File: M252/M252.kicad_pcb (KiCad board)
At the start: 2 copper layers, 50 x 40 mm, 20 parts, among them IC101 PIC16F1827-I/P, J101 UART, J102 PROG, J103 TRIP, Q101 10MHz, SW101 !MCLR

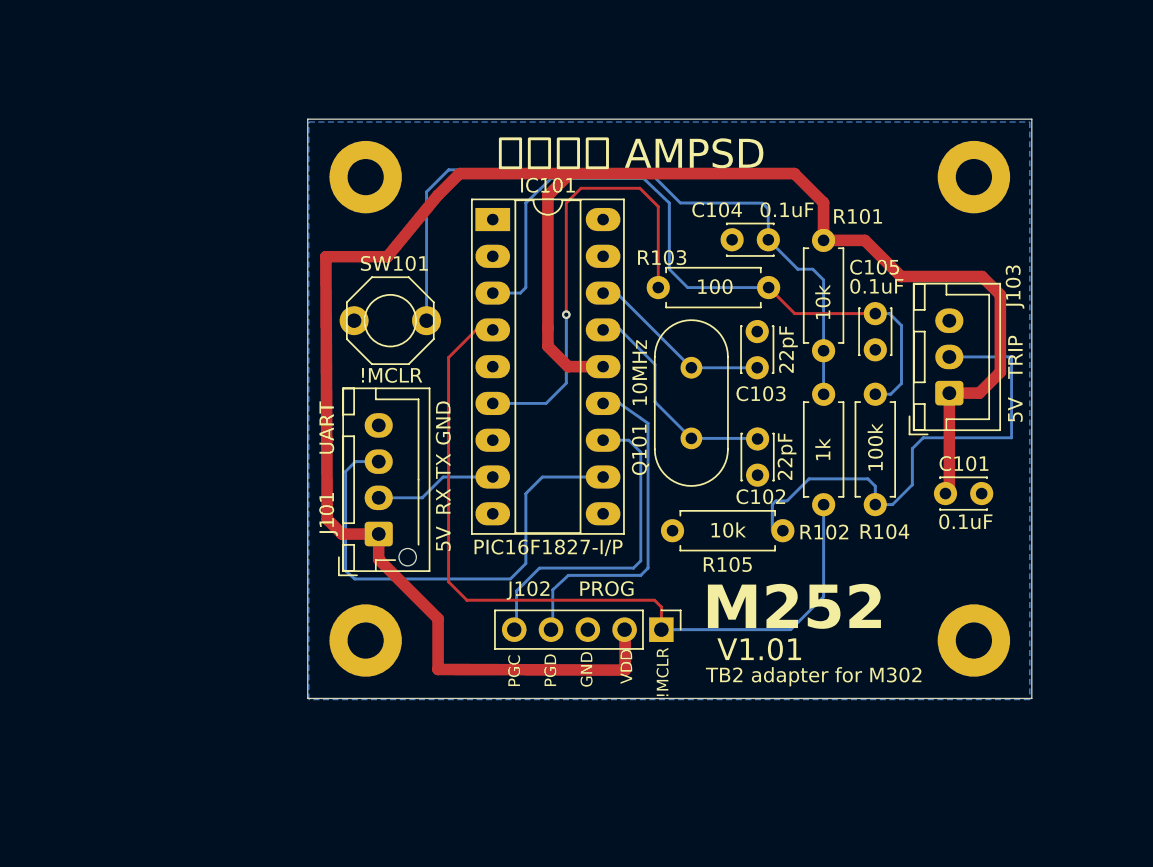
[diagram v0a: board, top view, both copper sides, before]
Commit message: UNO直結タイプ1st
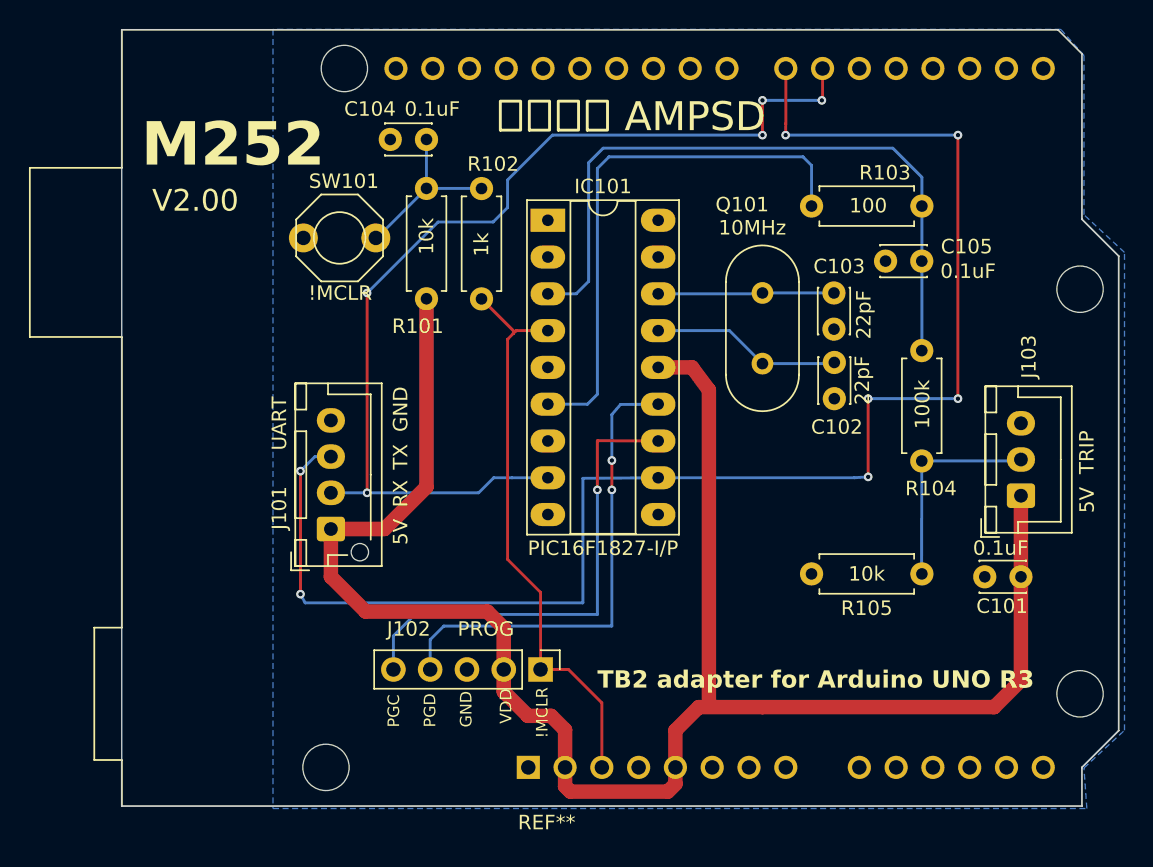
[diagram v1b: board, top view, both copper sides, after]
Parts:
- removed the REF** at (104.0, 96.0)
- removed the REF** at (104.0, 64.0)
- removed the REF** at (146.0, 64.0)
- removed the REF** at (146.0, 96.0)
- added REF**: Arduino_UNO_R3_WithMountingHoles, Module:Arduino_UNO_R3_WithMountingHoles, F.Cu at (115.2, 56.5)
- moved R101 29.6 mm to (108.2, 64.8), turned to -90 degrees
- moved R102 27.6 mm to (112.0, 72.4)
- moved C104 24.6 mm to (108.2, 61.4)
- moved R103 12.0 mm to (142.4, 66.0)
- moved R105 10.1 mm to (142.4, 91.4)
- moved J102 8.79 mm to (116.1, 98.0)
- moved J103 8.64 mm to (149.2, 86.0)
- moved C102 7.48 mm to (136.4, 76.8)
- moved C103 7.40 mm to (136.3, 72.0), turned to -90 degrees
- moved Q101 7.12 mm to (131.4, 72.0)
- moved SW101 6.70 mm to (102.2, 68.2)
- moved C101 5.75 mm to (146.8, 91.6), turned to 0 degrees
- moved C105 4.84 mm to (142.4, 69.8), turned to 180 degrees
- moved R104 4.40 mm to (142.4, 83.6)
- moved IC101 3.80 mm to (116.6, 67.0)
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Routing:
- net /TB2_TX: track 33.2 -> 105.5 mm, vias 0 -> 7
- net /TB2_RX: track 8.47 -> 70.9 mm, vias 0 -> 5
- net Net-(C104-Pad1): track 49.2 -> 12.1 mm
- net Net-(J103-Pin_2): track 33.8 -> 14.7 mm
- net Net-(IC101-RA5/~{MCLR}/VPP): track 54.8 -> 39.7 mm
- net Net-(IC101-RB6): track 22.6 -> 33.2 mm, vias 0 -> 1
- net +5V: track 136.5 -> 126.8 mm
- net Net-(IC101-RB7): track 23.5 -> 33.1 mm, vias 0 -> 2
- net Net-(IC101-RB0): track 31.0 -> 37.5 mm, vias 1 -> 0
- net Net-(IC101-RA6): track 15.3 -> 13.1 mm
- net Net-(IC101-RA7): track 12.8 -> 12.2 mm
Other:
- board size 50 x 40 mm -> 68.8 x 53.6 mm
- board text added: "TB2 adapter for Arduino UNO R3"
- board text added: "V2.00"
- board text removed: "TB2 adapter for M302"
- board text removed: "V1.01"
